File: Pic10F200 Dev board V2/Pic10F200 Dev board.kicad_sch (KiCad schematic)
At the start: 13 parts, among them J1 USB_C_Receptacle_PowerOnly_6P, J2 Conn_01x06_Pin, SW1 SW_Push, U1 PIC10F200-IOT

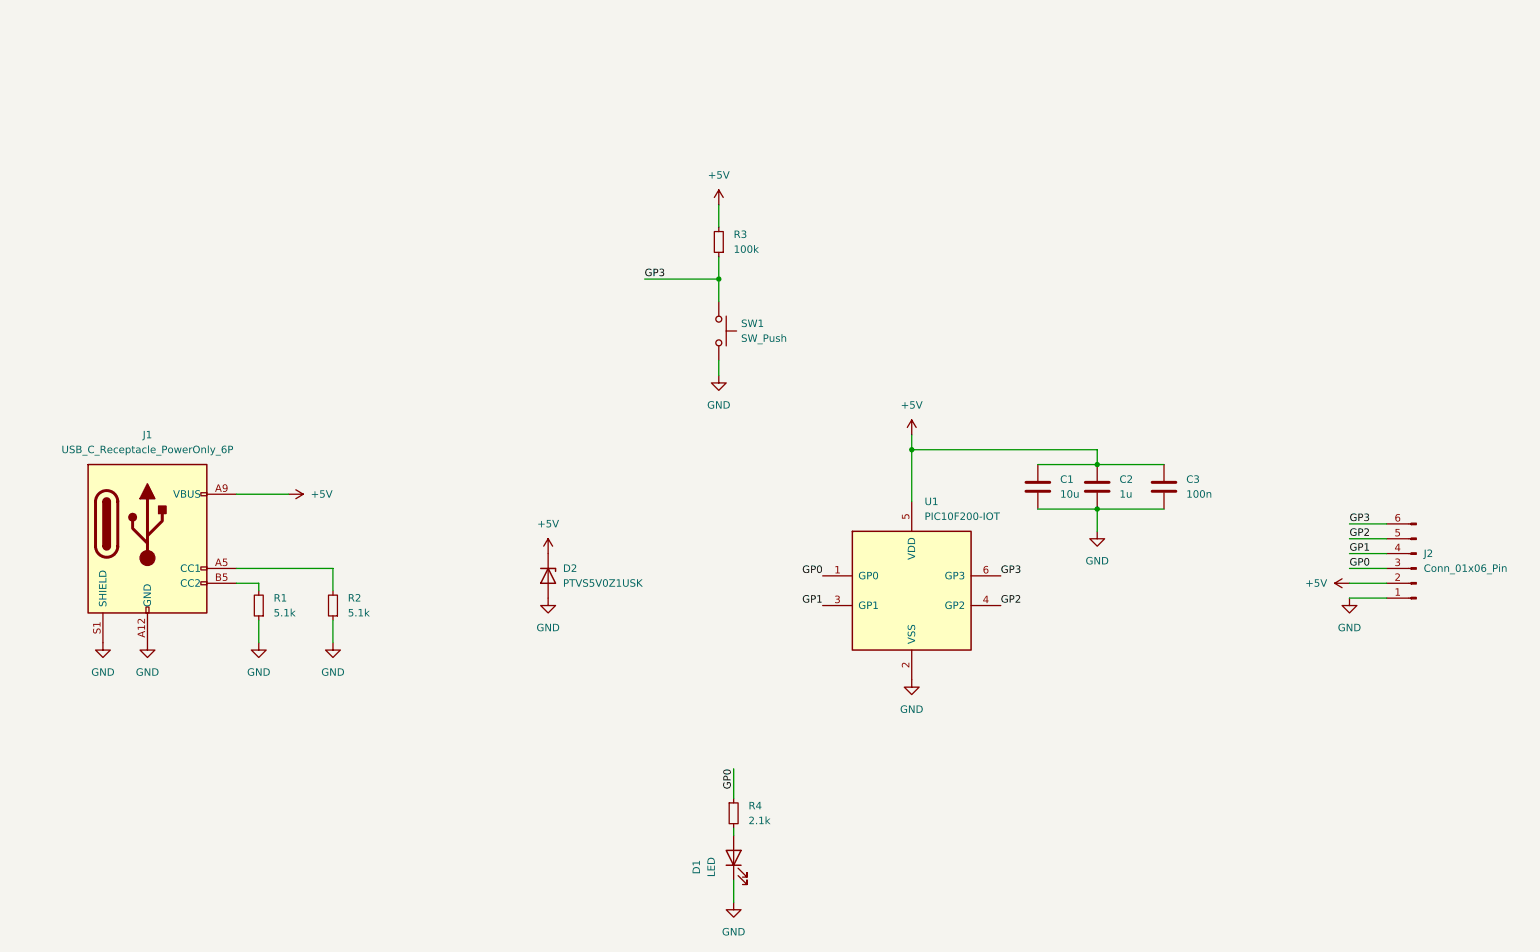
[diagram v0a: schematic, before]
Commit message: Cleaned Schematic and PCB layout
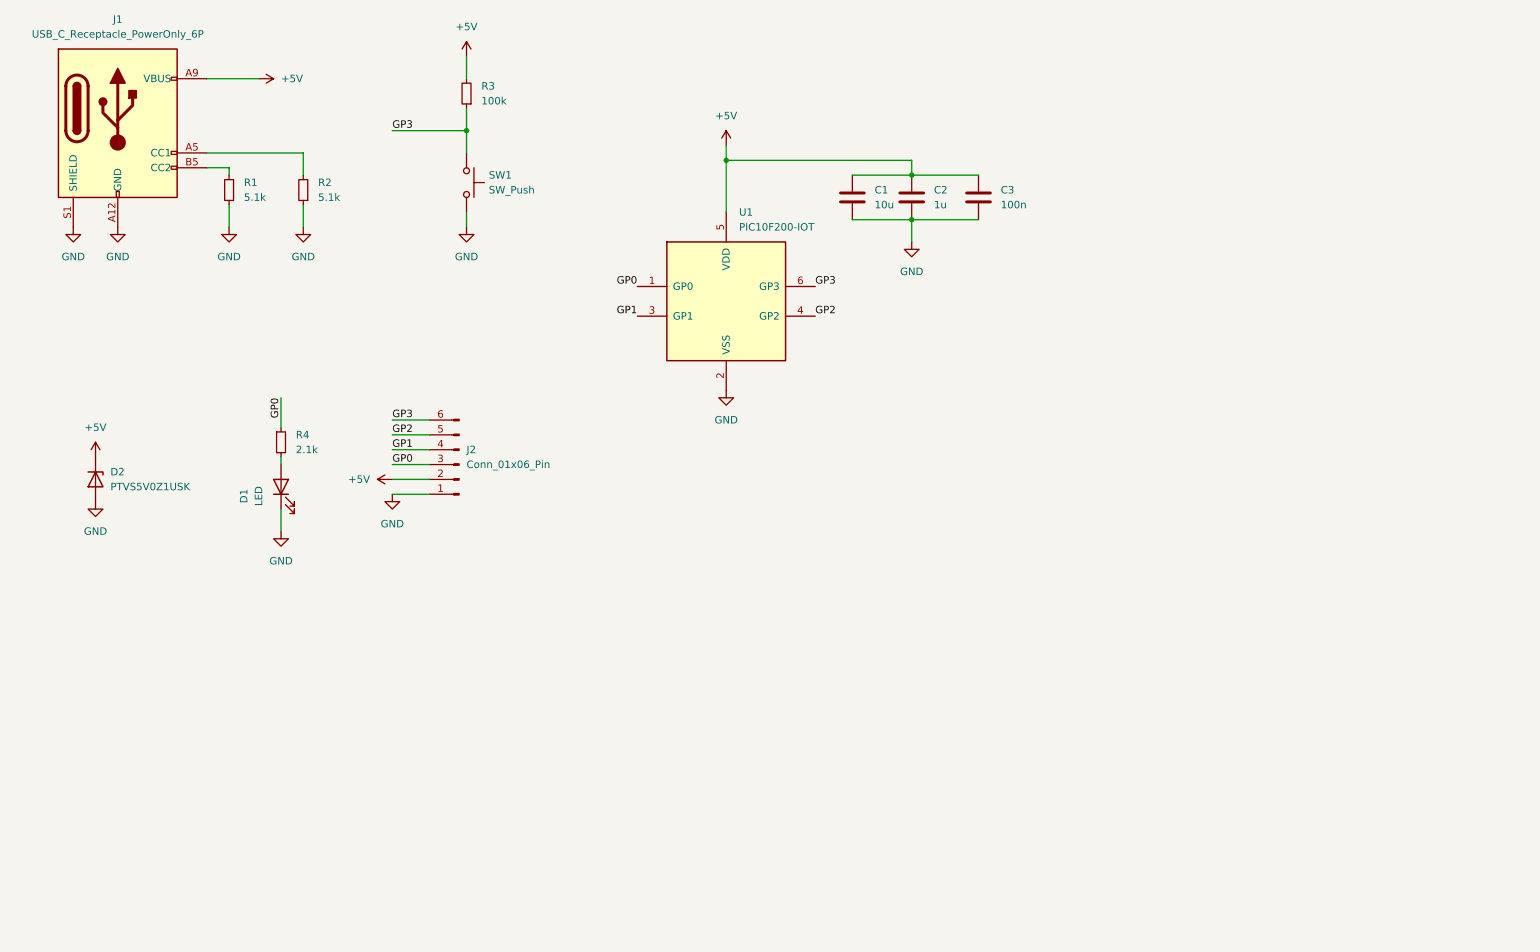
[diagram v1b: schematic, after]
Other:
- company: (none) -> Julien UHRY
- title: (none) -> PIC10F200 Dev Board
- moved on the sheet: C1, C2, C3, D1, D2, J1, J2, R1, R2, R3, R4, SW1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
